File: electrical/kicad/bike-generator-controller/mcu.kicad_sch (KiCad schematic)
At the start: 4 parts, among them J6 LiPo 1S / JST-PH 2.0 / PROV., U2 DFR0868 Beetle ESP32-C3

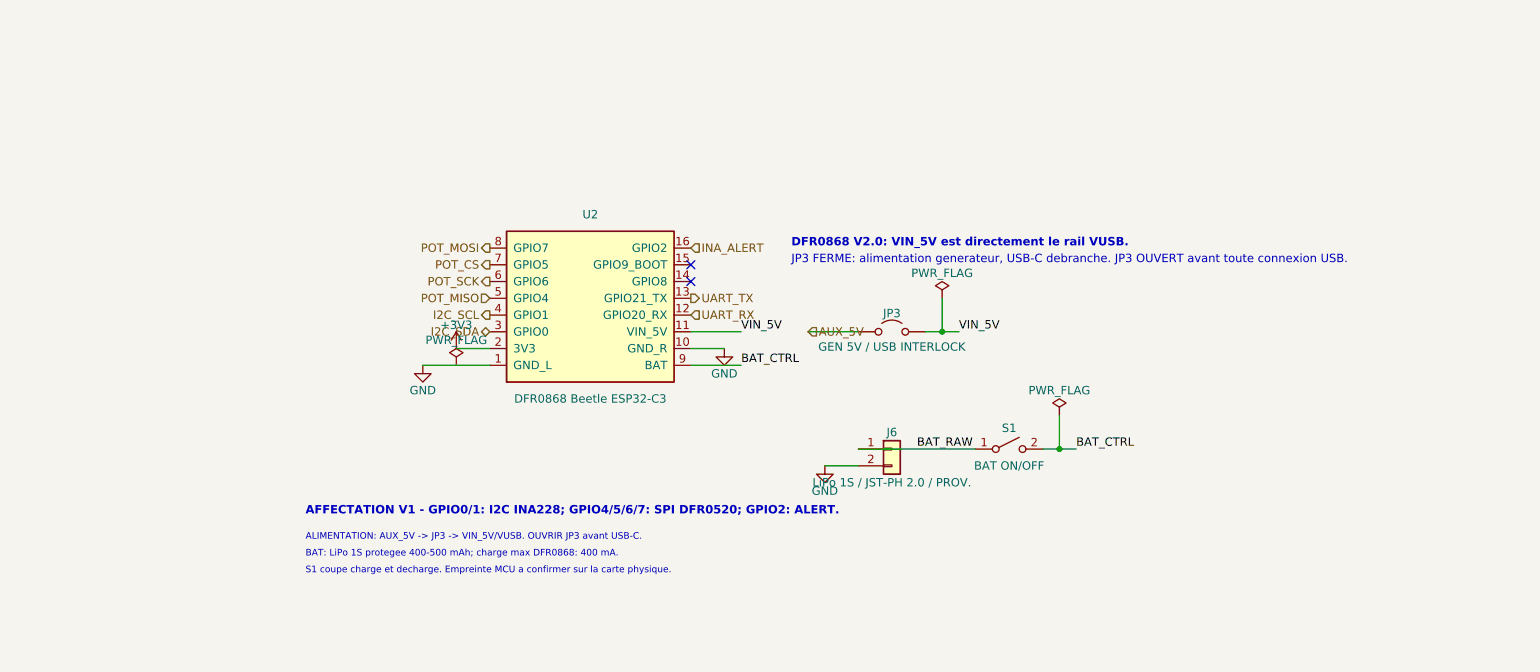
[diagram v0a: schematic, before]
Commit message: feat: establish controller PCB V1 design baseline
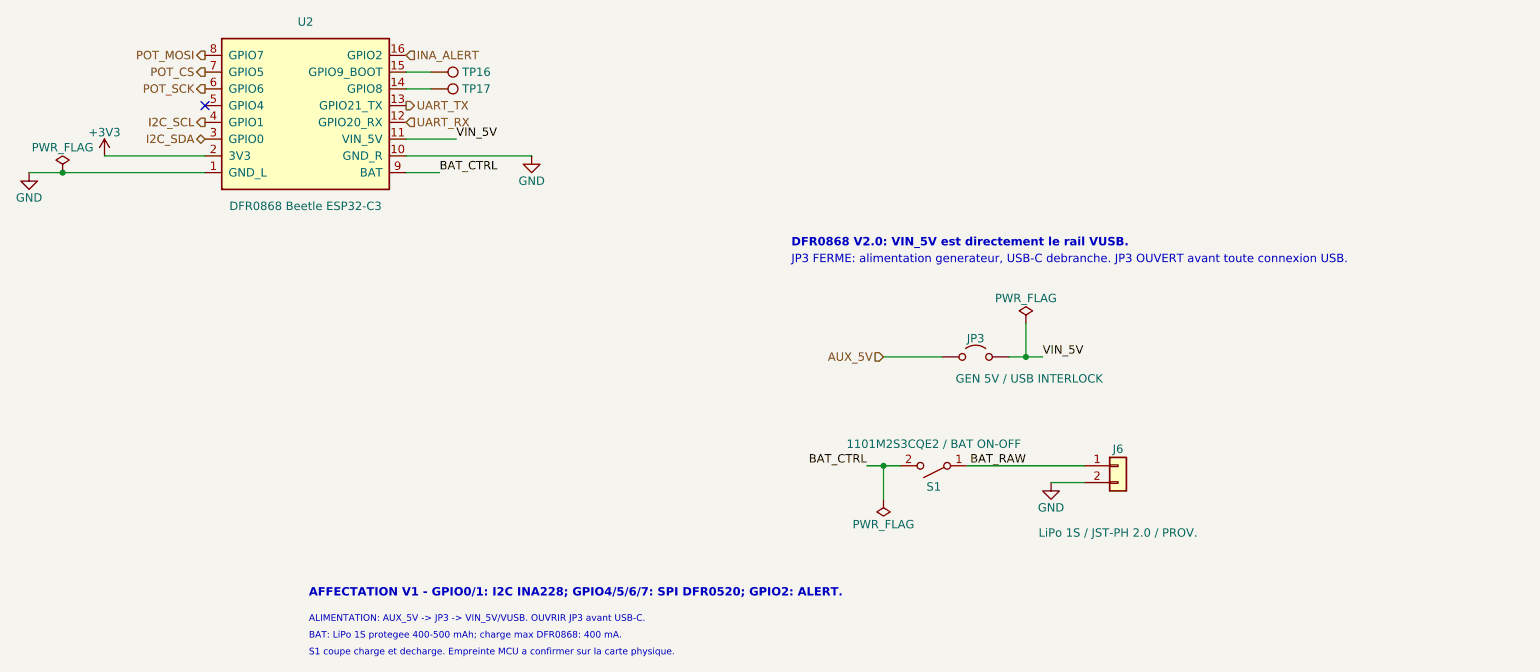
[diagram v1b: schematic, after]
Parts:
- added TP16, TP17: GND, TestPoint:TestPoint_Pad_D1.5mm, symbol Connector:TestPoint
- S1: value BAT ON/OFF -> 1101M2S3CQE2 / BAT ON-OFF; footprint (none) -> BikeGenerator:SW_1101M2S3CQE2; Contact Rating (none) -> 6 A @ 28 VDC; MPN (none) -> 1101M2S3CQE2; Manufacturer (none) -> C&K / Littelfuse; Physical Pad 3 (none) -> NC - unused throw
- U2: footprint (none) -> BikeGenerator:DFR0868_Beetle_ESP32-C3_V2_Socketed; MPN (none) -> DFR0868; Manufacturer (none) -> DFRobot
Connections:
- net at U2.14 (GPIO8): now also TP17.1
- net at U2.15 (GPIO9_BOOT): now also TP16.1
- net POT_MISO: no longer names the net of U2.5 (GPIO4)
- no-connect marks 2 -> 1
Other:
- moved on the sheet: J6, JP3, S1, U2
